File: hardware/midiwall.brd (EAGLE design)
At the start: 63.5 x 40.6 mm, 16 parts, among them IC1 PIC16F1825SO14

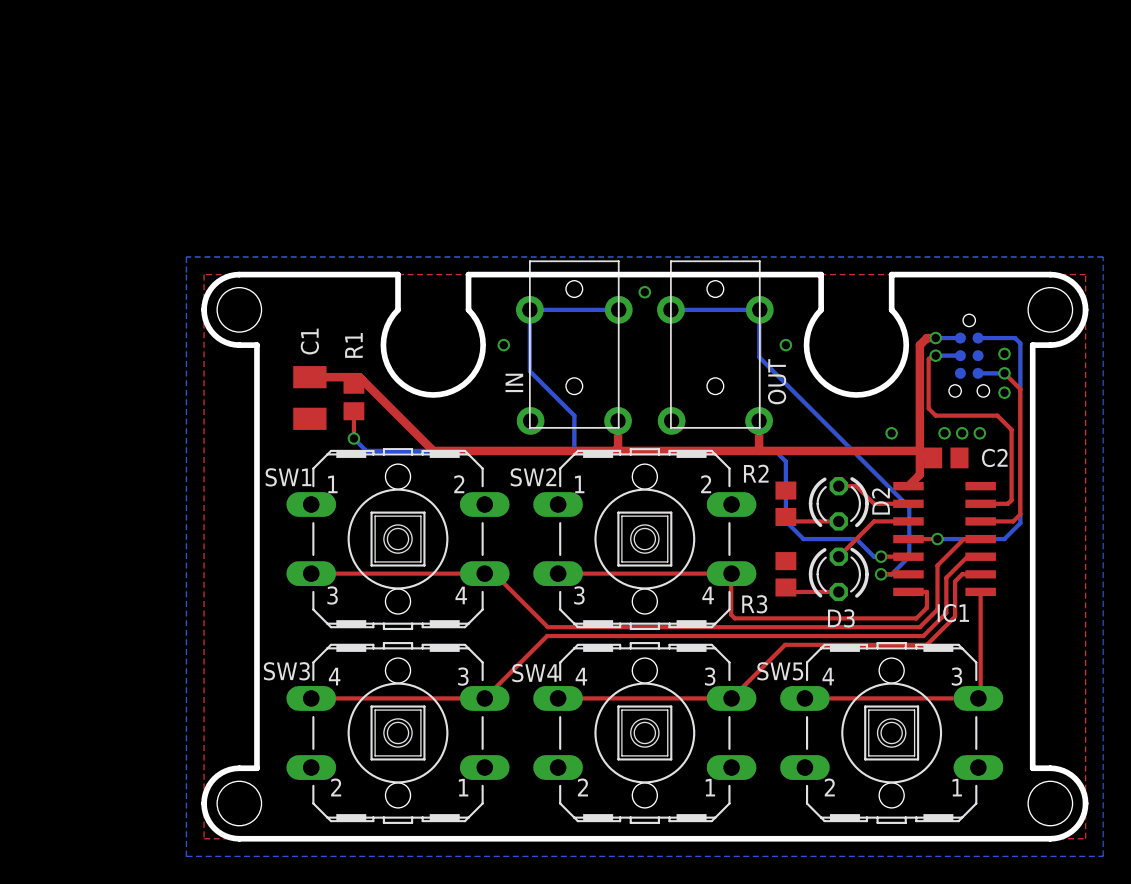
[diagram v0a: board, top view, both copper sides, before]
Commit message: assdadasadsaddas
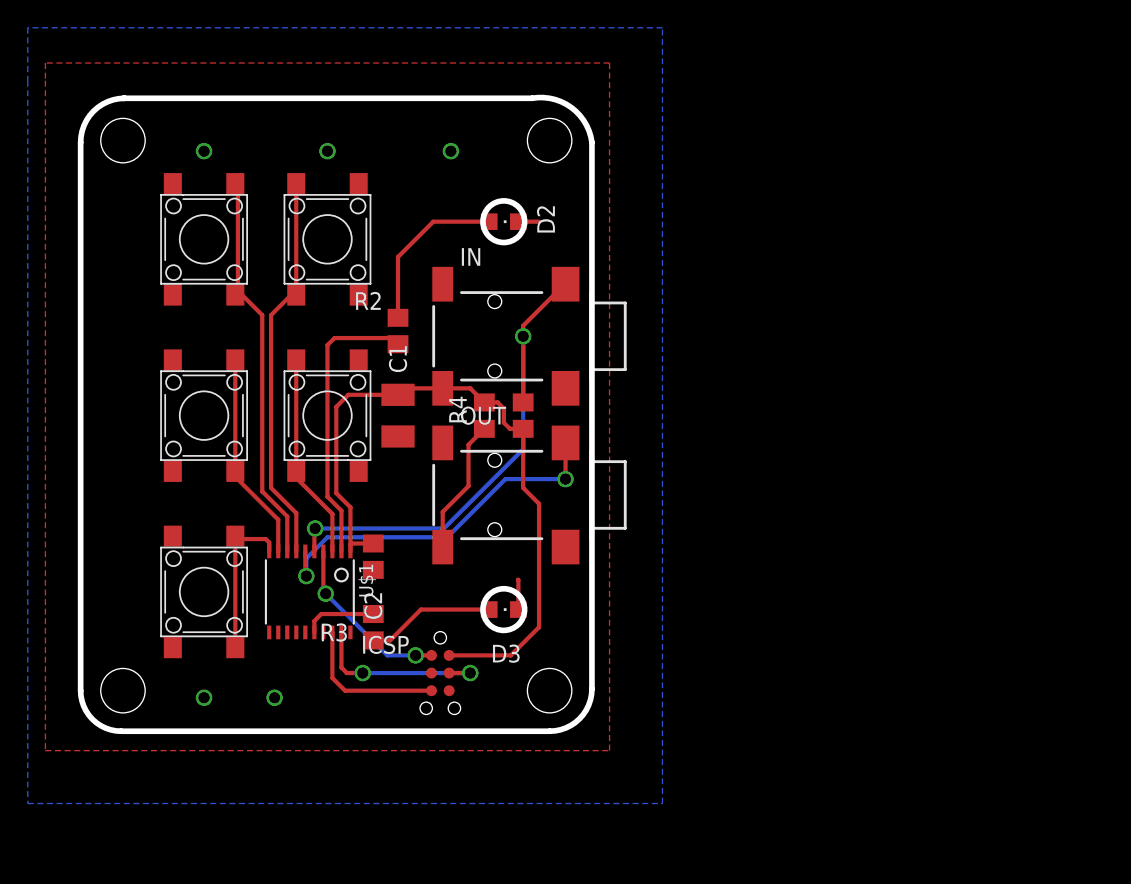
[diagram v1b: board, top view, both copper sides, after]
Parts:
- removed IC1: PIC16F1825SO14, jasons_stuff:SO14
- removed SW1, SW2, SW3, SW4, SW5: (no value), switch-omron:B3F-40XX
- added R4: (no value), rcl:R0805
- added U$1: PIC16F15345, jason_eagle6:TSSOP20
- added U$2, U$3, U$4, U$5, U$6: 6MMTACTSMT, jason_eagle6:6MMTACTSMT
- D2, D3: device led:LED3MM -> adafruit:CHIPLED_0805
- IN, OUT: value 3_5MM_PTH_MICRO -> 1503_02; device jason_eagle6:3_5MM_PTH_MICRO -> con-lumberg:1503_02
- moved ICSP 44.4 mm to (25.9, 17.0), flipped to the top
- moved C2 41.9 mm to (21.1, 22.9), turned to 270 degrees
- moved D2 31.5 mm to (30.5, 47.0)
- moved R2 30.6 mm to (22.9, 39.1)
- moved R3 30.0 mm to (21.1, 17.8), turned to 90 degrees
- moved D3 24.3 mm to (30.5, 19.1)
- moved OUT 16.0 mm to (36.8, 27.3), turned to 270 degrees
- moved R1 12.3 mm to (31.9, 33.0), turned to 270 degrees
- moved C1 6.48 mm to (22.9, 33.0)
- moved IN 2.29 mm to (36.8, 38.7), turned to 270 degrees
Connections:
- new net N$3: OUT.3, R4.1
- net +5V: now also R4.2, U$1.1; no longer IC1.1, OUT.3
- net GND: now also D2.C, D3.C, U$1.20, U$2.2, U$2.3, U$3.2, U$3.3, U$4.2, U$4.3, U$5.2, U$5.3, U$6.2, U$6.3; no longer IC1.14, R2.1, R3.1, SW1.1, SW1.2, SW2.1, SW2.2, SW3.1, SW3.2, SW4.1, SW4.2, SW5.1, SW5.2
- net KEY1: now also U$1.3, U$6.1, U$6.4; no longer IC1.10, SW3.3, SW3.4
- net KEY2: now also U$1.7, U$5.1, U$5.4; no longer IC1.7, SW2.3, SW2.4
- net KEY3: now also U$1.8, U$4.1, U$4.4; no longer IC1.9, SW4.3, SW4.4
- net KEY4: now also U$1.9, U$3.1, U$3.4; no longer IC1.11, SW1.3, SW1.4
- net KEY5: now also U$1.10, U$2.1, U$2.4; no longer IC1.8, SW5.3, SW5.4
- net LED1: now also R2.2, U$1.2; no longer D2.A, IC1.2
- net LED2: now also R3.2, U$1.16; no longer D3.A, IC1.3
- net N$1: now also D2.A, R2.1; no longer D2.K, R2.2
- net N$2: now also D3.A, R3.1; no longer D3.K, R3.2
- net PGC: now also U$1.18; no longer IC1.12
- net PGD: now also U$1.19; no longer IC1.13
- net RX: now also U$1.5; no longer IC1.5, IN.2A
- net TX: now also U$1.6; no longer IC1.6, OUT.2A
- net VPP: now also U$1.4; no longer IC1.4
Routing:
- net KEY1: track 53.9 -> 14.9 mm
- net KEY4: track 54.3 -> 15.4 mm
- net RX: track 65.9 -> 37.0 mm
- net +5V: track 66.7 -> 50.4 mm, vias 1 -> 0
- net LED1: track 5.55 -> 20.9 mm
- net VPP: track 24.7 -> 12.6 mm, vias 1 -> 2
- net N$3: track 0.00 -> 9.76 mm
- net KEY5: track 20.2 -> 11.3 mm
- net N$1: track 3.94 -> 12.0 mm
- net KEY3: track 35.6 -> 28.4 mm
- net TX: track 33.2 -> 26.7 mm, vias 1 -> 2
- net PGD: track 20.0 -> 13.5 mm, vias 1 -> 2
- net N$2: track 3.94 -> 9.27 mm
- net PGC: track 15.6 -> 10.8 mm, vias 1 -> 0
- net KEY2: track 32.5 -> 28.4 mm
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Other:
- board size 63.5 x 40.6 mm -> 36.8 x 45.6 mm
- board text removed: "MIDIWALL V4"
- board text removed: "hotchk155/2022"
